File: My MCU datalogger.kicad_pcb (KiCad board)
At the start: 2 copper layers, 47.6 x 30.5 mm, 29 parts, among them J1 Conn_01x04_Male, J2 Conn_01x09_Male, J3 Conn_01x04_Male, J4 Conn_02x03_Odd_Even, U1 24LC1025, U2 DS1307Z, U3 24LC1025, U4 ATMEGA328P-AU, Y1 32.768 KHz, Y2 16 MHz

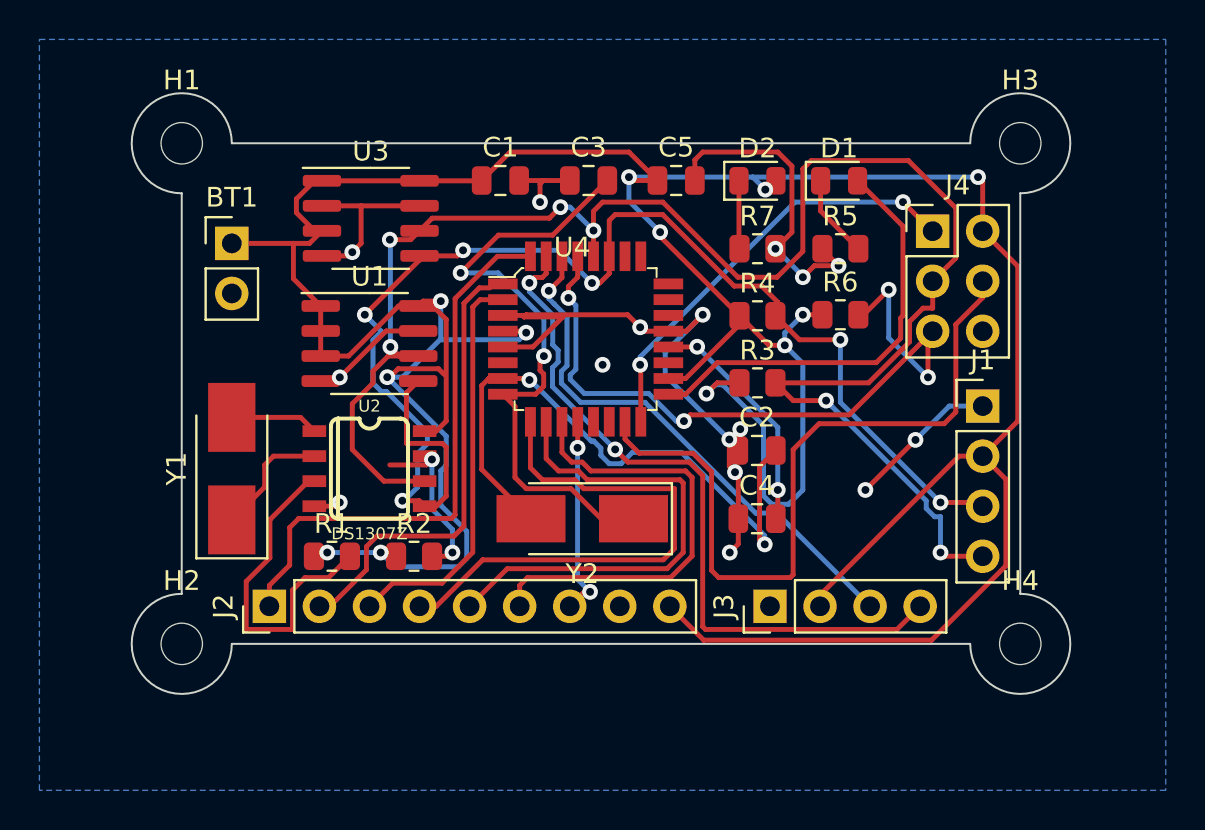
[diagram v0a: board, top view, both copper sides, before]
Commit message: Finalized
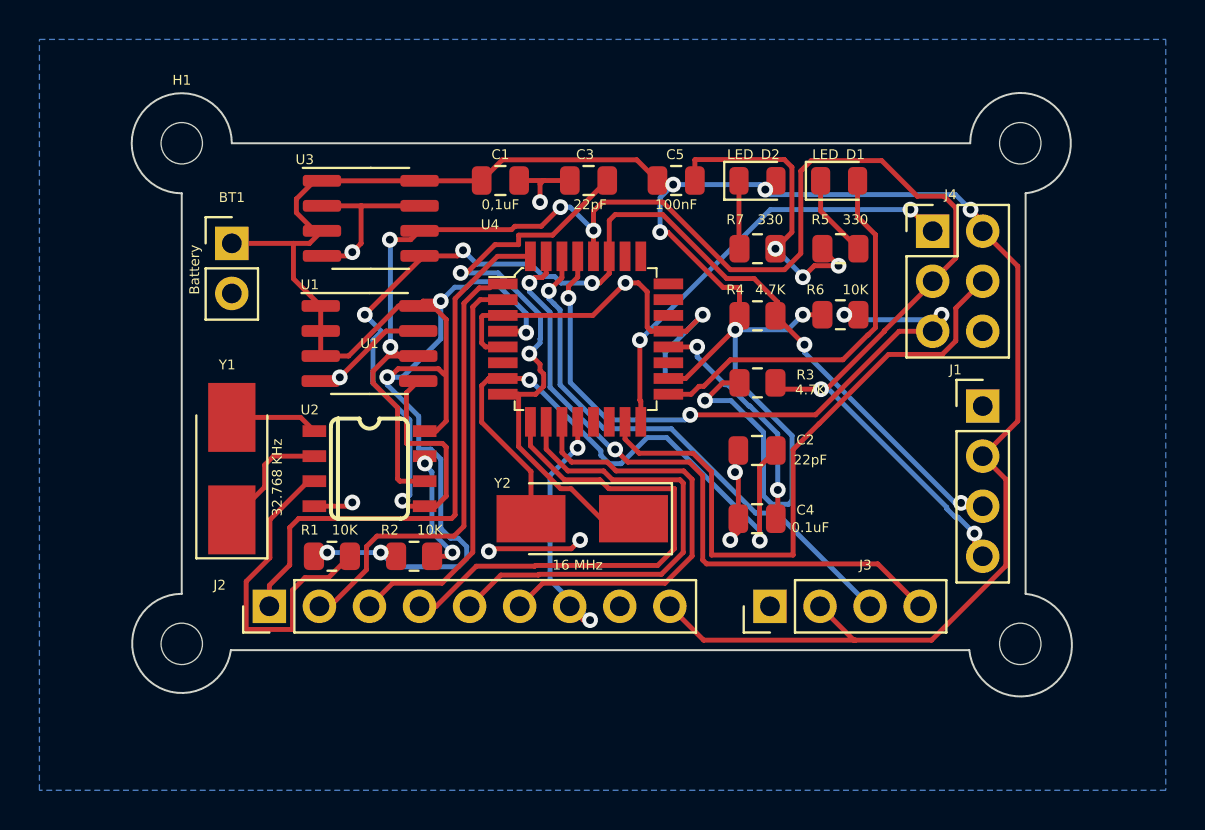
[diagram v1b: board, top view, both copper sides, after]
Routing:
- net /Vcc: track 197.1 -> 184.8 mm
- net GND: track 77.2 -> 66.0 mm, vias 16 -> 13
- net /SCK: track 89.4 -> 83.4 mm
- net /MOSI: track 37.9 -> 33.8 mm
- net /TX: track 36.6 -> 33.5 mm
- net /RESET: track 37.6 -> 34.6 mm
- net /D8: track 9.93 -> 12.8 mm
- net Net-(R2-Pad2): track 8.96 -> 6.21 mm
- net /SDA: track 67.5 -> 65.0 mm
- net Net-(D1-Pad2): track 22.0 -> 19.7 mm
- net /D7: track 23.2 -> 22.4 mm
- net /D5: track 27.3 -> 26.6 mm
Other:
- board size 47.6 x 30.5 mm -> 47.7 x 30.6 mm
